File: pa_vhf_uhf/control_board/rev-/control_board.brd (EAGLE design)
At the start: 160 x 100 mm, 0 parts

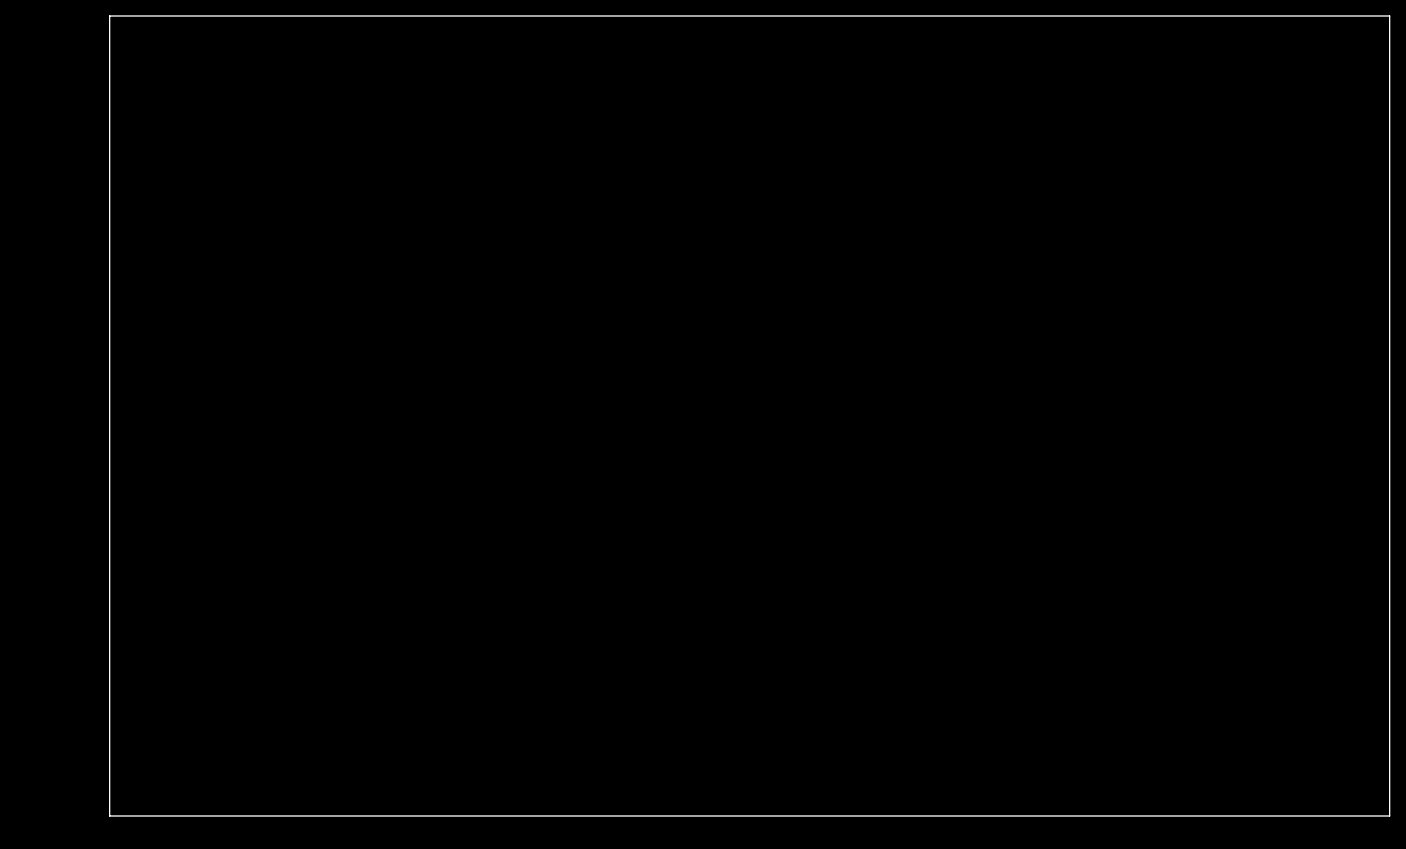
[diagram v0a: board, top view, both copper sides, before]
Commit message: minor updates to control board.
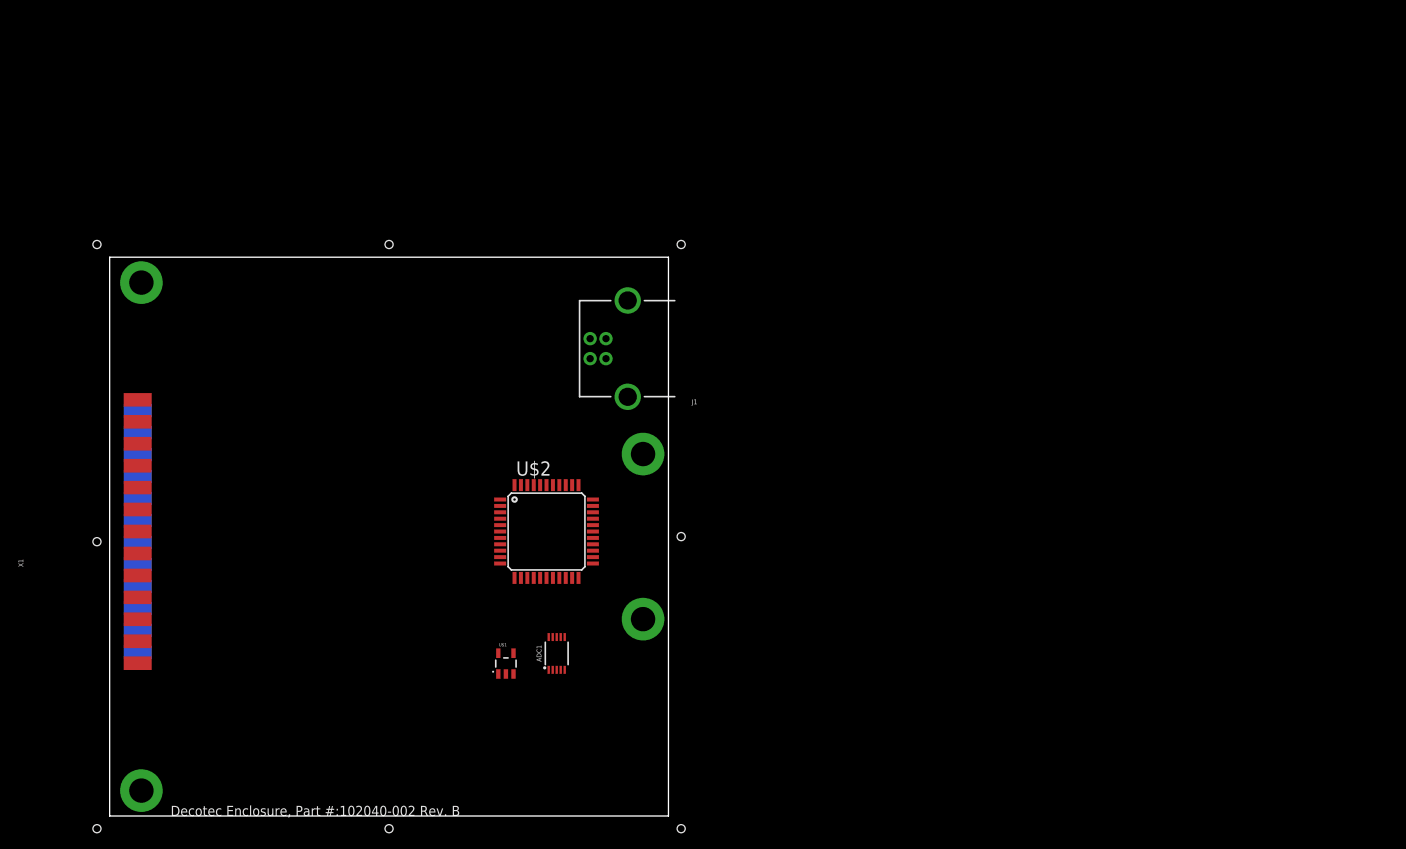
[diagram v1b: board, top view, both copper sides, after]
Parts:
- added ADC1: ADS1115, vtgs:MSOP10
- added J1: USB_B_PTH, SparkFun-Connectors:USB-B-PTH
- added U$1: SPX3819M5_5V, kj4qlp:SOT23-5
- added U$2: ATMEGA32U4-AU, adafruit:TQFP44
- added U$3: DECOTEC_102040-002B, vtgs:DECOTEC_102040-002B
- added X1: (no value), SparkFun-Retired:M25D
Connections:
- new net GND: J1.GND
- new net VBUS: J1.VBUS
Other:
- board size 160 x 100 mm -> 69.8 x 69.8 mm
